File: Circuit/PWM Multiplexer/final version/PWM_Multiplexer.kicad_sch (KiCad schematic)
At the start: 71 parts, among them J1 JST connector, Q1 S8050, Q10 S8050, Q11 S8050, Q12 S8050, Q13 S8050, Q14 S8050, Q2 S8050, Q3 S8050, Q4 S8050, Q5 S8050, Q6 S8050, Q7 S8050, Q8 S8050, Q9 S8050, U1 PC817, U2 PC817, U3 PC817, U4 PC817, U5 L7805, U6 74HC137, U7 74HC137

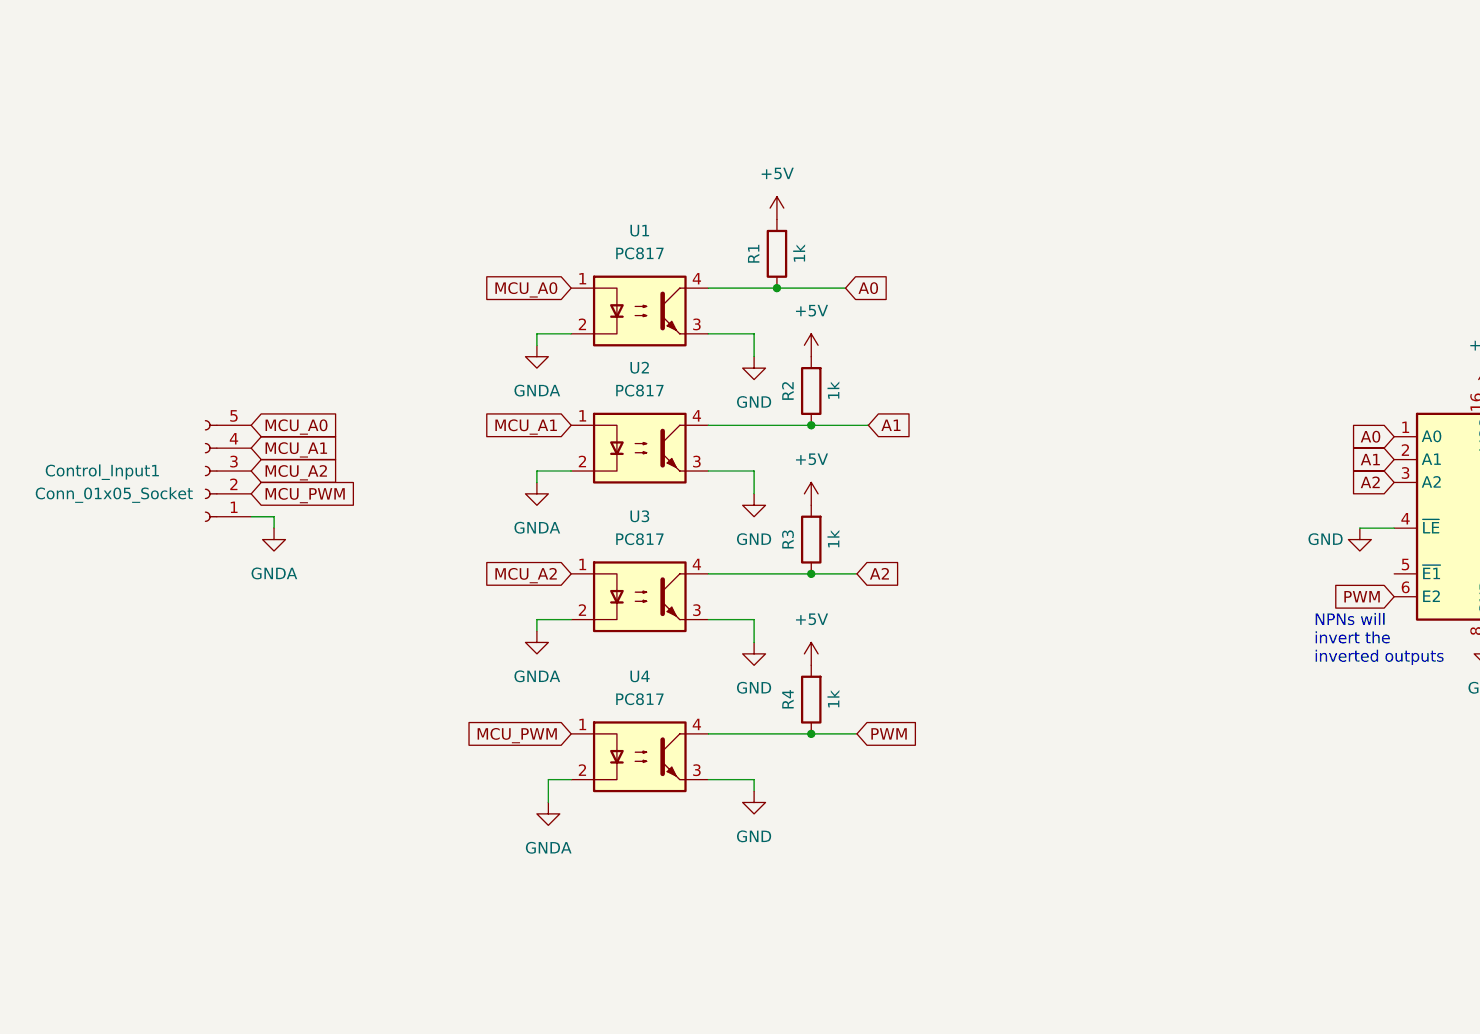
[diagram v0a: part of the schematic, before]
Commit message: further development in esp32-cam
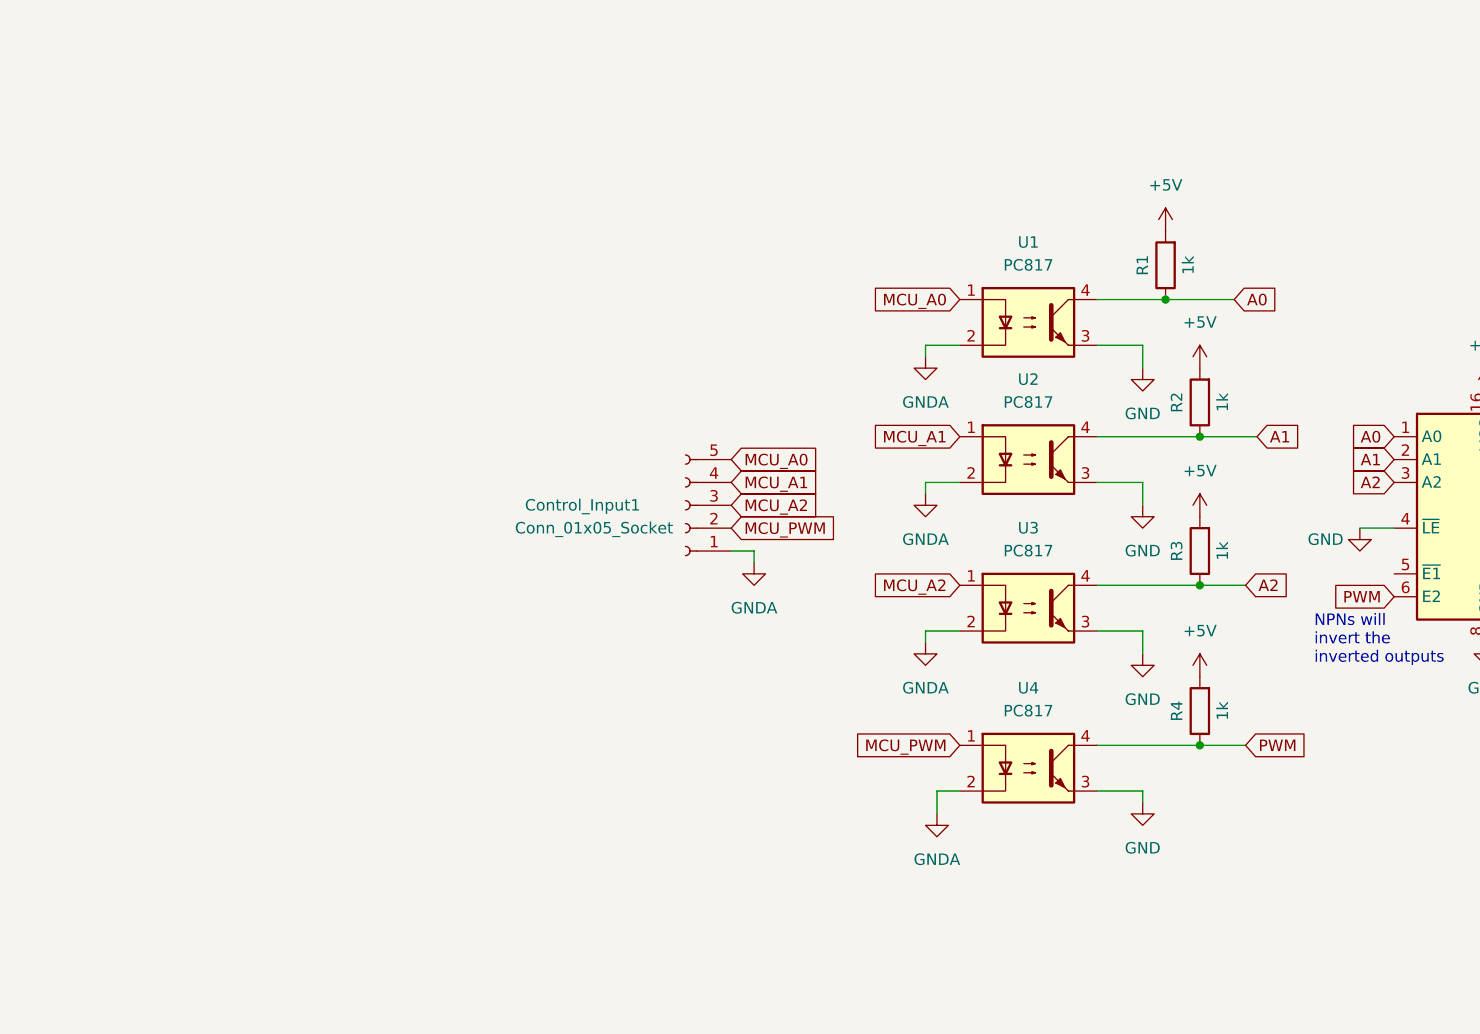
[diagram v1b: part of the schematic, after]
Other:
- moved on the sheet: Control_Input1, R1, R2, R3, R4, U1, U2, U3, U4
